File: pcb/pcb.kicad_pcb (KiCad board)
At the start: 2 copper layers, 49.7 x 21.4 mm, 2 parts, among them U1 ESP32-S3-WROOM-1(N8R8)

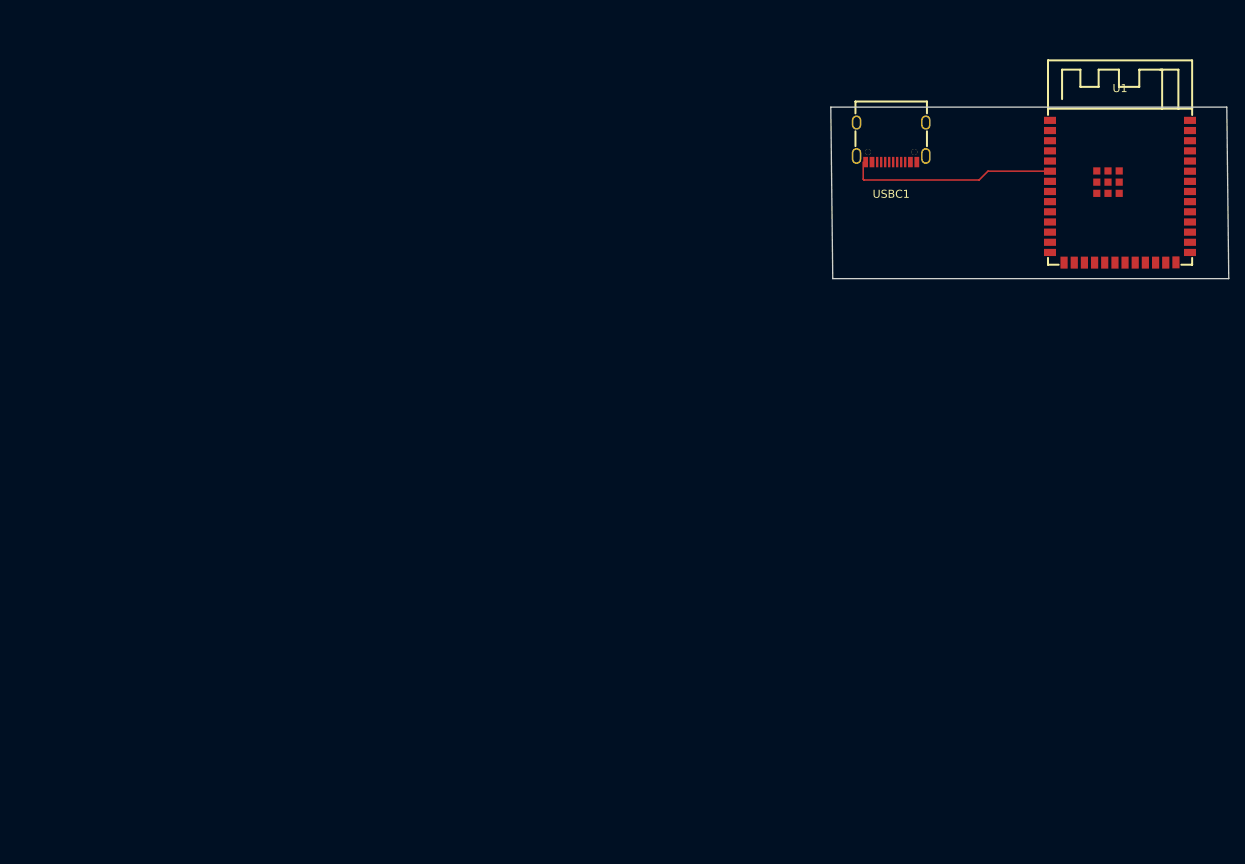
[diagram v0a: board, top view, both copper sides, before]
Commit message: Much more work
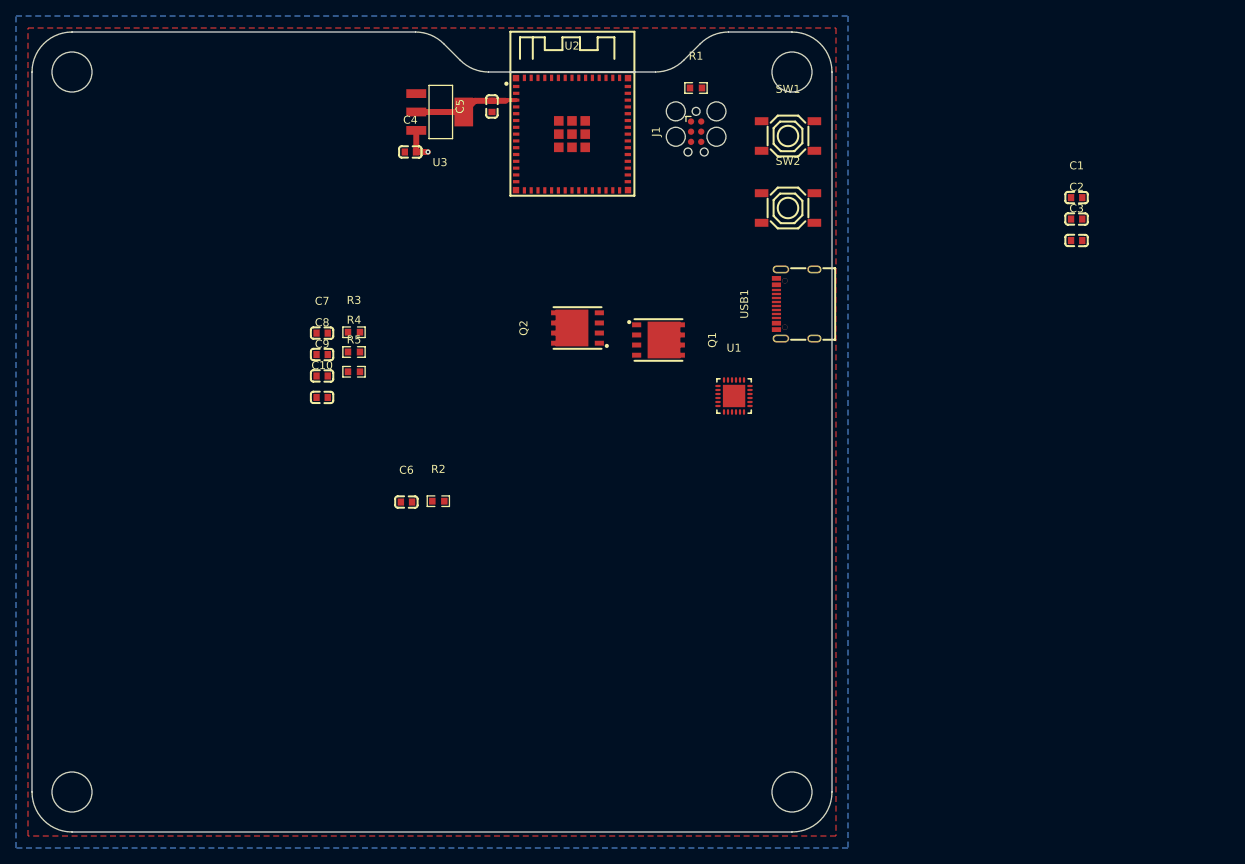
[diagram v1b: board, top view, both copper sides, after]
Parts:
- removed USBC1: TYPE-C-31-M-12, EasyEDA:USB-C_SMD-TYPE-C-31-M-12
- added C1: 1uF, EasyEDA:C0603, F.Cu at (180.6, 70.7)
- added C10: 1uF, EasyEDA:C0603, F.Cu at (86.3, 95.7)
- added C2: 22uF, EasyEDA:C0603, F.Cu at (180.6, 73.4)
- added C3: 0.1uF, EasyEDA:C0603, F.Cu at (180.6, 76.1)
- added C4: 0.1uF, EasyEDA:C0603, F.Cu at (97.3, 65.0)
- added C5: 22uF, EasyEDA:C0603, F.Cu at (107.5, 59.3)
- added C6: 4.7nF, EasyEDA:C0603, F.Cu at (96.8, 108.8)
- added C7: 0.1uF, EasyEDA:C0603, F.Cu at (86.3, 87.6)
- added C8: 1uF, EasyEDA:C0603, F.Cu at (86.3, 90.3)
- added C9: 1uF, EasyEDA:C0603, F.Cu at (86.3, 93.0)
- added J1: TagConnect_TC2030, Connector:Tag-Connect_TC2030-IDC-FP_2x03_P1.27mm_Vertical, F.Cu at (133.0, 62.5)
- added Q1: STL60P4LLF6, EasyEDA:POWERFLAT-8_L5.2-W6.0-P1.27-LS6.2-BL, F.Cu at (128.3, 88.5)
- added Q2: STL60P4LLF6, EasyEDA:POWERFLAT-8_L5.2-W6.0-P1.27-LS6.2-BL, F.Cu at (118.2, 87.0)
- added R1: 10kΩ, EasyEDA:R0603, F.Cu at (133.0, 57.0)
- added R2: 1MΩ, EasyEDA:R0603, F.Cu at (100.8, 108.7)
- added R3: 100kΩ, EasyEDA:R0603, F.Cu at (90.2, 87.5)
- added R4: 22kΩ, EasyEDA:R0603, F.Cu at (90.2, 90.0)
- added R5: 100Ω, EasyEDA:R0603, F.Cu at (90.2, 92.5)
- added SW1: TS-1187A-B-A-B, EasyEDA:SW-SMD_4P-L5.1-W5.1-P3.70-LS6.5-TL-2, F.Cu at (144.5, 63.0)
- added SW2: TS-1187A-B-A-B, EasyEDA:SW-SMD_4P-L5.1-W5.1-P3.70-LS6.5-TL-2, F.Cu at (144.5, 72.0)
- added U2: ESP32-S3-MINI-1-N8, EasyEDA:BULETM-SMD_ESP32-S3-MINI-1-N8, F.Cu at (117.5, 62.8)
- added U3: AMS1117-3.3, EasyEDA:SOT-223-3_L6.5-W3.4-P2.30-LS7.0-BR, F.Cu at (101.0, 60.0)
- added USB1: TYPEC-304A-ACP16L, EasyEDA:USB-C-SMD_XUNPU_TYPEC-304A-ACP16L, F.Cu at (145.4, 84.0)
- U1: value ESP32-S3-WROOM-1(N8R8) -> STUSB4500QTR; footprint EasyEDA:WIRELM-SMD_ESP32-S3-WROOM-1 -> EasyEDA:QFN-24_L4.0-W4.0-P0.50-BL-EP2.8
- moved U1 54.6 mm to (137.8, 95.5)
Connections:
- U1 pad 10: unconnected-(U1-IO17-Pad10) -> GND
- U1 pad 16: unconnected-(U1-IO46-Pad16) -> VBUS_EN_SNK
- U1 pad 22: unconnected-(U1-IO14-Pad22) -> GND
- U1 pad 23: unconnected-(U1-IO21-Pad23) -> VREG_2V7
- U1 pad 24: unconnected-(U1-IO47-Pad24) -> VUNREG
- U1 pad 25: unconnected-(U1-IO48-Pad25) -> GND
- U1 pad 6: Net-(U1-IO6) -> unconnected-(U1-RESET-Pad6)
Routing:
- net Net-(U1-IO6): track 26.0 -> 0.00 mm
- net +3V3_MCU: track 0.00 -> 13.4 mm
- net +5V: track 0.00 -> 4.21 mm, vias 0 -> 1
- added copper zone on In2.Cu, net +5V
- added copper zone on B.Cu, net GND
- added copper zone on F.Cu, net GND
- added copper zone on In1.Cu, net GND
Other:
- board size 49.7 x 21.4 mm -> 100 x 100 mm
- copper layers 2 -> 4
